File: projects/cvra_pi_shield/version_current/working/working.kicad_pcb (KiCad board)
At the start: 4 copper layers, 65 x 56 mm, 50 parts, among them J1 Conn_02x20_Odd_Even, J10 Conn_01x04, J11 0530470210, J12 Conn_01x03, J2 Conn_01x04, J3 Conn_01x04, J4 0530470210, J5 Conn_01x05, J6 Conn_01x07, J7 0530471410, J8 Conn_01x04, J9 Conn_01x04, Q1 DMP3099L, SW1 DIP SPST 100MA 6V, U1 MCP2515-xST, U2 MAX3051, U3 DS3231, U4 PCA9685BS, U5 TPS5430DDA, Y1 20Mhz

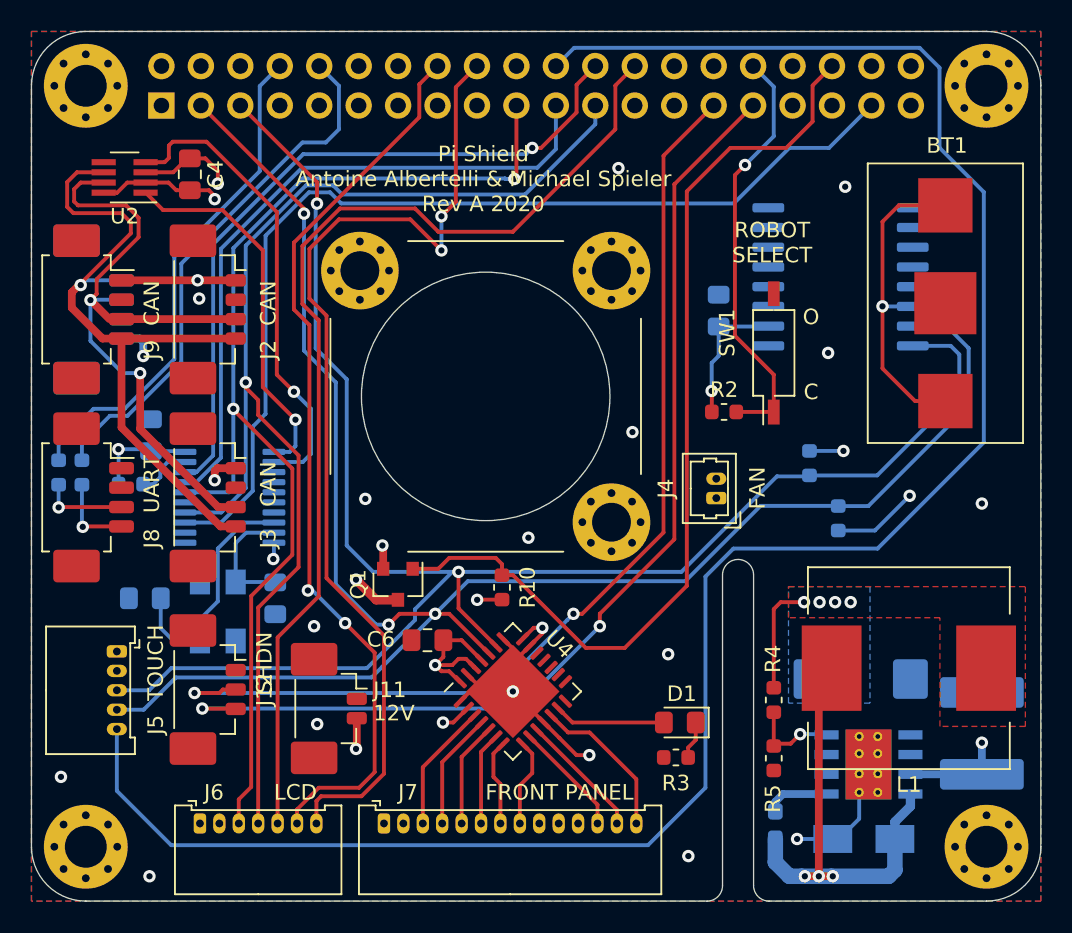
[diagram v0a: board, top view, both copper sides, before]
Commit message: updated all projects from src
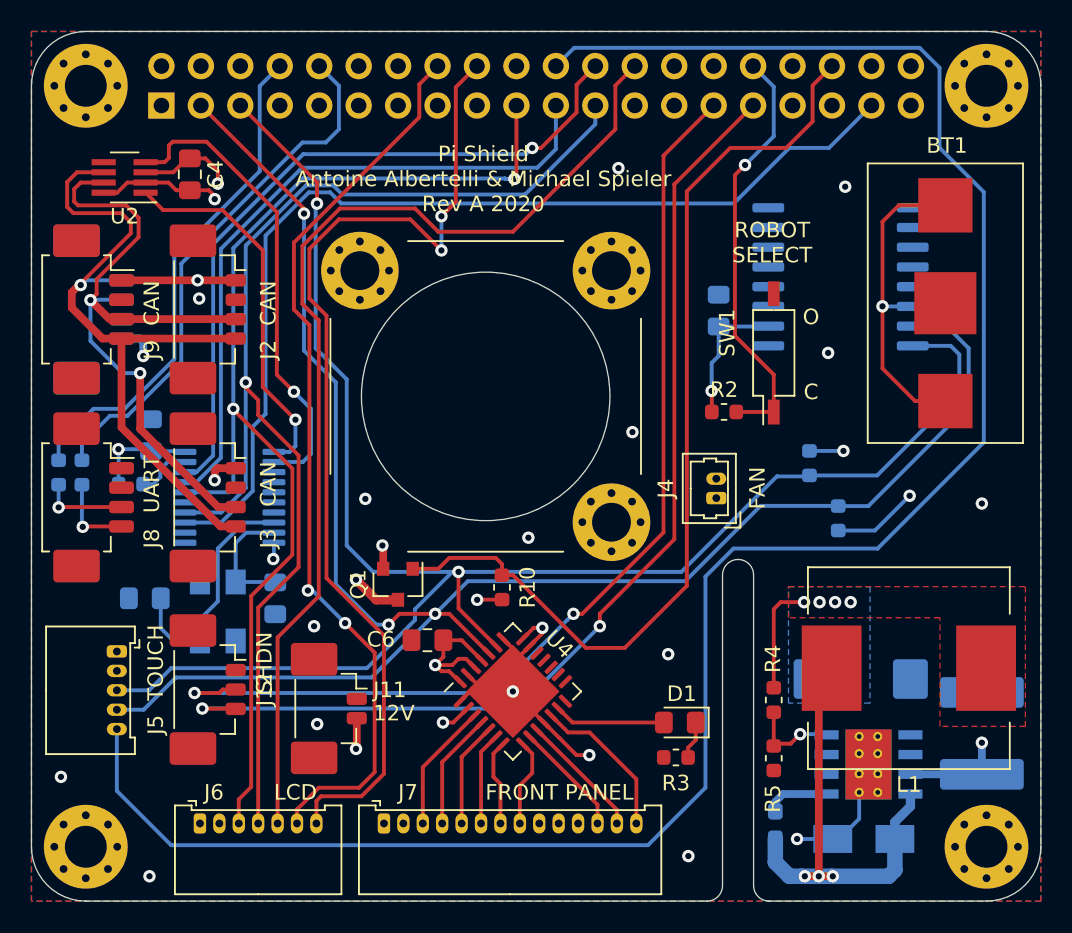
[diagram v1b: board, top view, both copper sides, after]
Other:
- net class Default added: clearance 0.15, trace_width 0.25, via_dia 0.8, via_drill 0.4

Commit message: some generations
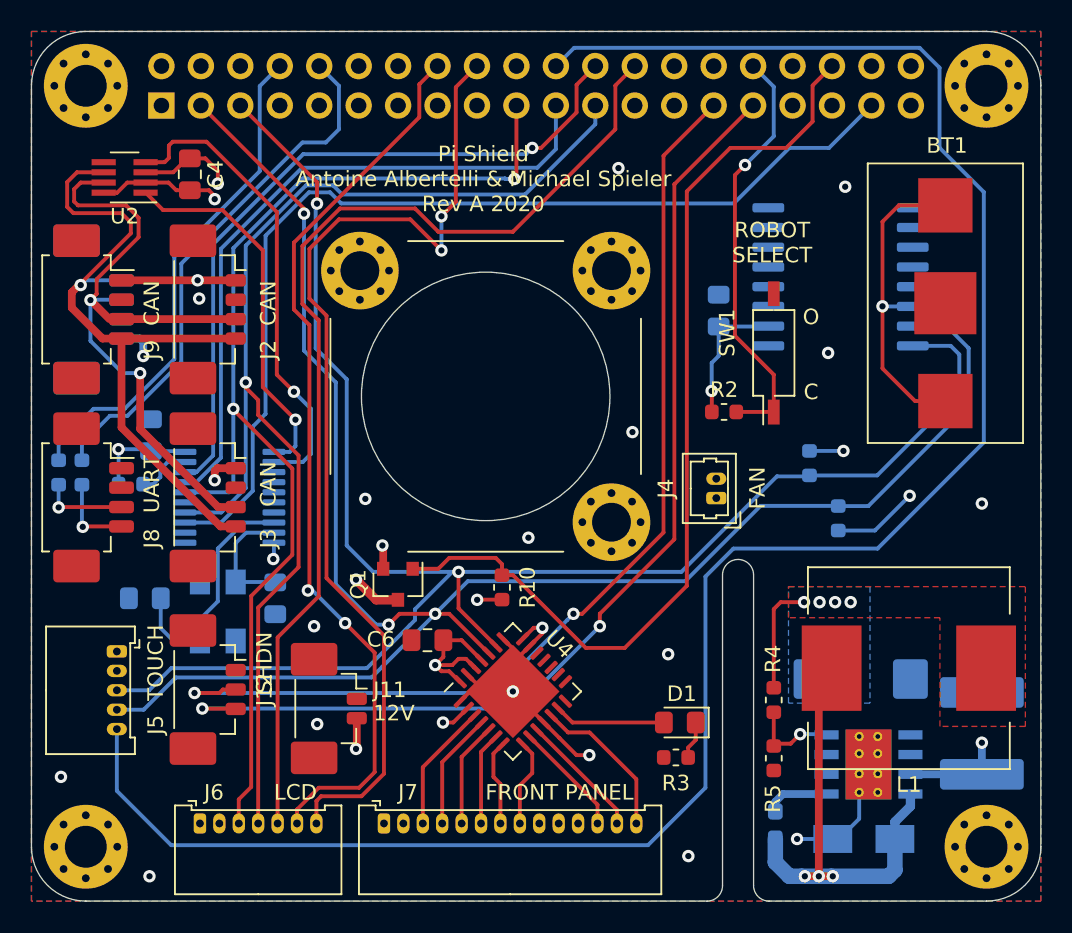
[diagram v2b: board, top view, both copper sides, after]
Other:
- net class Default removed
